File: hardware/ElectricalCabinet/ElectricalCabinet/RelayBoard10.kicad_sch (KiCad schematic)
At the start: 0 parts

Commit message: Further wiring updates
Populated 6100 Bus
Corrected number of relay boards
Added 110v outputs to relay boards and noted light positon
Uploaded light scheme to documents folder
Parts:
- added C10: 0.1uF, Capacitor_SMD:C_0805_2012Metric, symbol Device:C
- added D73, D74, D75, D76, D77, D78, D79, D80: LED, LED_SMD:LED_0805_2012Metric, symbol Device:LED
- added J20: Screw_Terminal_01x06, TerminalBlock:TerminalBlock_MaiXu_MX126-5.0-06P_1x06_P5.00mm, symbol Connector:Screw_Terminal_01x06
- added J21: Screw_Terminal_01x09, TerminalBlock:TerminalBlock_MaiXu_MX126-5.0-09P_1x09_P5.00mm, symbol Connector:Screw_Terminal_01x09
- added K73, K74, K75, K76, K77, K78, K79, K80: G3MB-202P DC5, TrafficLightLibrary:G3MB_202P_DC5, symbol TrafficLightLibrary:G3MB-202P_DC5
- added R73, R74, R75, R76, R77, R78, R79, R80: 1kΩ, Resistor_SMD:R_0805_2012Metric, symbol Device:R
- added U11: TPIC6B595N, TrafficLightLibrary:TPIC6B595N, symbol TrafficLightLibrary:TPIC6B595N
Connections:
- new net: D79.1 (K), R79.1
- new net: D73.2 (A), D74.2 (A), D75.2 (A), D76.2 (A), D77.2 (A), D78.2 (A), D79.2 (A), D80.2 (A), K73.3, K74.3, K75.3, K76.3, K77.3, K78.3, K79.3, K80.3
- new net: J21.9 (Pin_9), K73.1, K74.1, K75.1, K76.1, K77.1, K78.1, K79.1, K80.1
- new net: J21.4 (Pin_4), K76.2
- new net: K76.4, R76.2, U11.7 (DRAIN3)
- new net: D80.1 (K), R80.1
- new net: K80.4, R80.2, U11.17 (DRAIN7)
- new net: D75.1 (K), R75.1
- new net: D76.1 (K), R76.1
- new net: J20.1 (Pin_1), U11.18 (SEROUT)
- new net: C10.1, J20.2 (Pin_2), U11.10 (GND), U11.11 (GND), U11.19 (GND), U11.9 (~{G})
- new net: J20.3 (Pin_3), U11.13 (SRCK)
- new net: J20.4 (Pin_4), U11.12 (RCK)
- new net: C10.2, J20.6 (Pin_6), U11.2 (VCC), U11.8 (~{SRCLR})
- new net: K79.4, R79.2, U11.16 (DRAIN6)
- new net: K75.4, R75.2, U11.6 (DRAIN2)
- new net: D73.1 (K), R73.1
- new net: J21.5 (Pin_5), K77.2
- new net: K77.4, R77.2, U11.14 (DRAIN4)
- new net: J21.6 (Pin_6), K78.2
- new net: K78.4, R78.2, U11.15 (DRAIN5)
- new net: J21.2 (Pin_2), K74.2
- new net: K74.4, R74.2, U11.5 (DRAIN1)
- new net: J21.8 (Pin_8), K80.2
- new net: J21.1 (Pin_1), K73.2
- new net: K73.4, R73.2, U11.4 (DRAIN0)
- new net: D78.1 (K), R78.1
- new net: D77.1 (K), R77.1
- new net: J21.3 (Pin_3), K75.2
- new net: J21.7 (Pin_7), K79.2
- new net: D74.1 (K), R74.1
- new net SERIN: J20.5 (Pin_5), U11.3 (SERIN)
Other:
- note added: "RELAY MODULE 10"

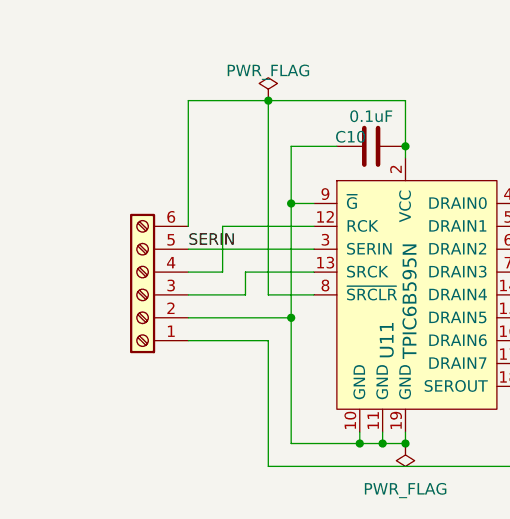
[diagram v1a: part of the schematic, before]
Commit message: Electrical Cabinet done
Electrical Cabinet done, let me know if there are any changes or mistakes.
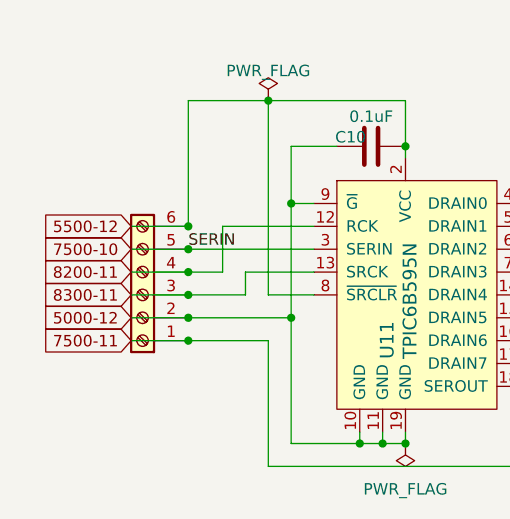
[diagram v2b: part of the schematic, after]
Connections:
- net 7500-11: now reaches J20.1 (Pin_1), U11.18 (SEROUT)
- net 5000-12: now reaches C10.1, J20.2 (Pin_2), U11.10 (GND), U11.11 (GND), U11.19 (GND), U11.9 (~{G})
- net 8300-11: now reaches J20.3 (Pin_3), U11.13 (SRCK)
- net 8200-11: now reaches J20.4 (Pin_4), U11.12 (RCK)
- net 5500-12: now reaches C10.2, J20.6 (Pin_6), U11.2 (VCC), U11.8 (~{SRCLR})
- net SERIN renamed 7500-10
